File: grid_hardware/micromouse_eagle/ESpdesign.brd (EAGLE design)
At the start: 89.8 x 61 mm, 8 parts

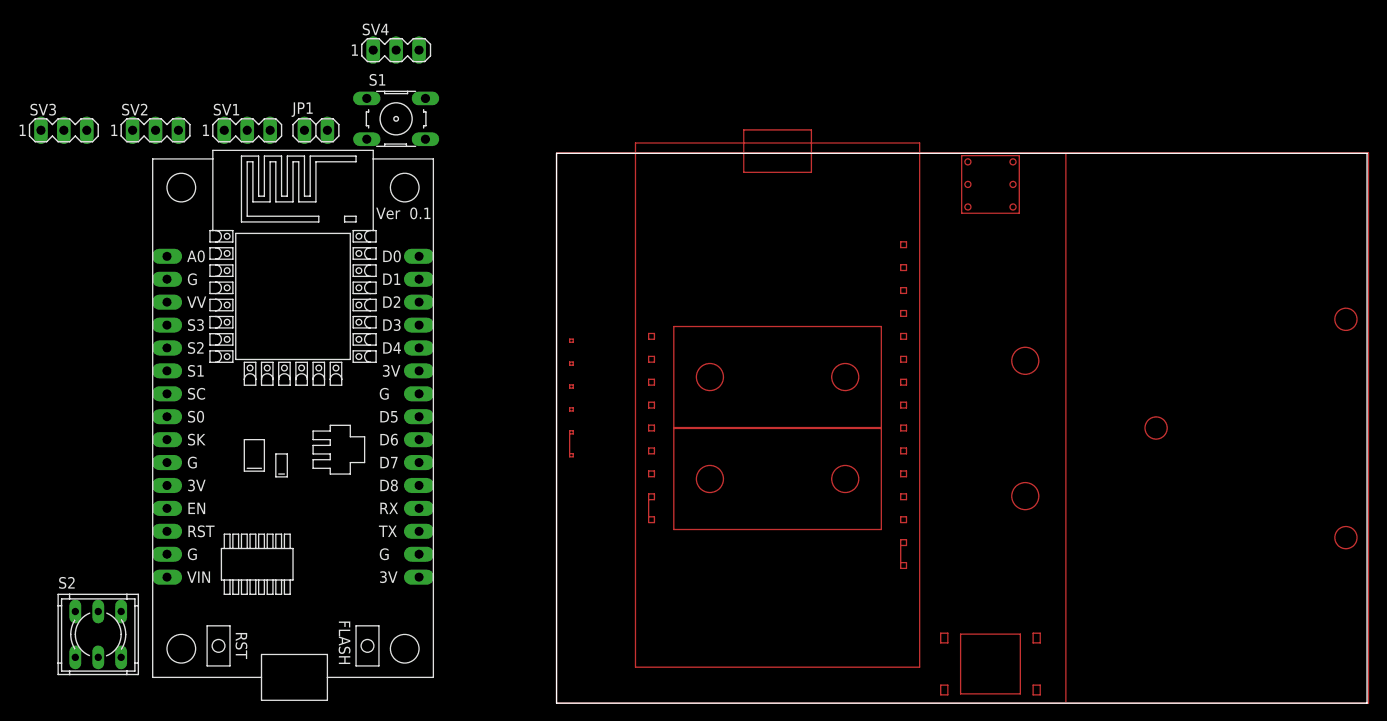
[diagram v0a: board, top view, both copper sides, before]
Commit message: brd continue
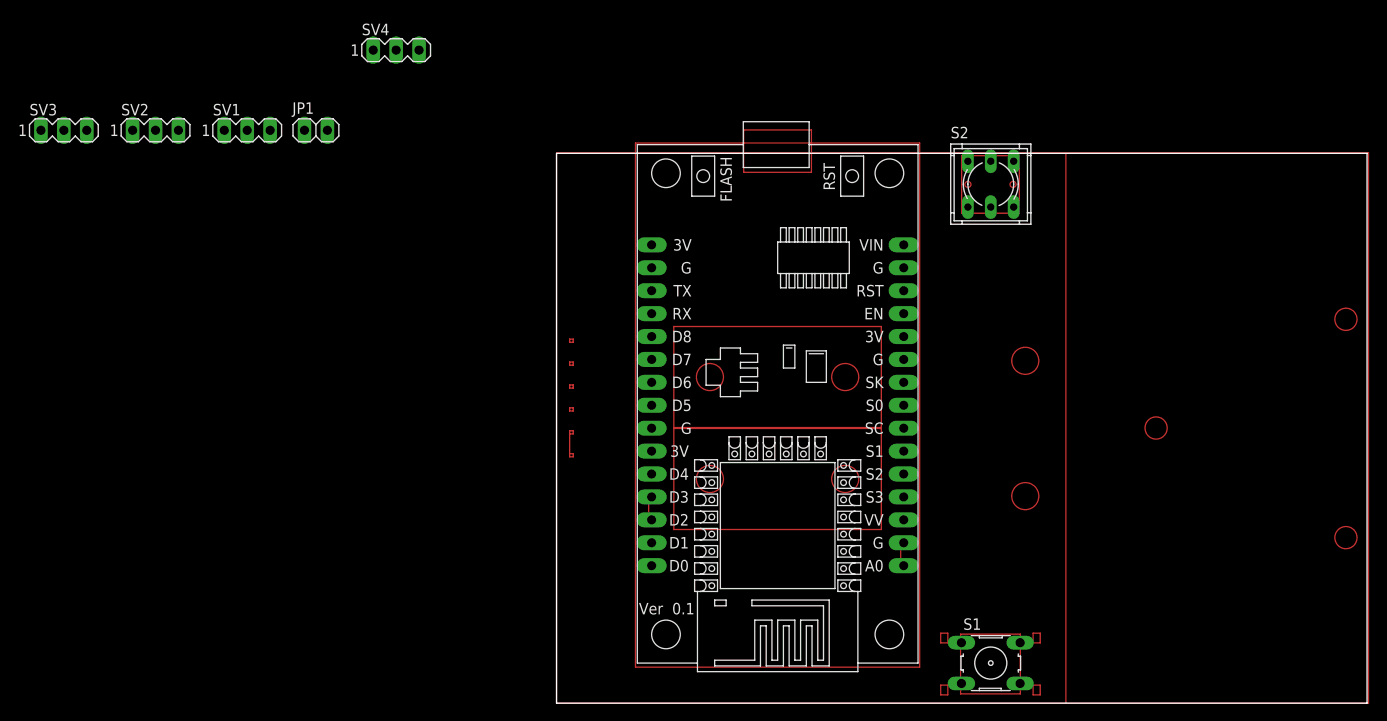
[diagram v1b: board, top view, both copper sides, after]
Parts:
- moved S2 110.8 mm to (48.1, 57.5)
- moved S1 89.4 mm to (48.1, 4.45)
- moved U$1 53.7 mm to (24.5, 33.0), turned to 180 degrees
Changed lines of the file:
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@@
 <attribute name="VALUE" x="-29.21" y="60.325" size="1.27" layer="27"/>
 </element>
-<element name="S1" library="switch-omron" library_urn="urn:adsk.eagle:library:377" package="B3F-10XX" package3d_urn="urn:adsk.eagle:package:27496/1" value="" x="-17.78" y="64.77" smashed="yes">
-<attribute name="MF" value="" x="0" y="0" size="1.778" layer="27" display="off"/>
-<attribute name="MPN" value="B3F-1000" x="0" y="0" size="1.778" layer="27" display="off"/>
-<attribute name="NAME" x="-20.828" y="68.453" size="1.27" layer="25" ratio="10"/>
-<attribute name="OC_FARNELL" value="176432" x="0" y="0" size="1.778" layer="27" display="off"/>
-<attribute name="OC_NEWARK" value="36M3542" x="0" y="0" size="1.778" layer="27" display="off"/>
-<attribute name="POPULARITY" value="72" x="0" y="0" size="1.778" layer="27" display="off"/>
-<attribute name="VALUE" x="-20.828" y="59.69" size="1.27" layer="27" ratio="10"/>
+<element name="S1" library="switch-omron" library_urn="urn:adsk.eagle:library:377" package="B3F-10XX" package3d_urn="urn:adsk.eagle:package:27496/1" value="" x="48.133" y="4.445" smashed="yes">
+<attribute name="MF" value="" x="65.913" y="-60.325" size="1.778" layer="27" display="off"/>
+<attribute name="MPN" value="B3F-1000" x="65.913" y="-60.325" size="1.778" layer="27" display="off"/>
+<attribute name="NAME" x="45.085" y="8.128" size="1.27" layer="25" ratio="10"/>
+<attribute name="OC_FARNELL" value="176432" x="65.913" y="-60.325" size="1.778" layer="27" display="off"/>
+<attribute name="OC_NEWARK" value="36M3542" x="65.913" y="-60.325" size="1.778" layer="27" display="off"/>
+<attribute name="POPULARITY" value="72" x="65.913" y="-60.325" size="1.778" layer="27" display="off"/>
+<attribute name="VALUE" x="45.085" y="-0.635" size="1.27" layer="27" ratio="10"/>
 </element>
-<element name="S2" library="switch-misc-edited" package="9077-2" package3d_urn="urn:adsk.eagle:package:27425/1" value="9077-2" x="-50.8" y="7.62" smashed="yes">
-<attribute name="NAME" x="-55.245" y="12.7" size="1.27" layer="25" ratio="10"/>
-<attribute name="POPULARITY" value="1" x="0" y="0" size="1.778" layer="27" display="off"/>
-<attribute name="VALUE" x="-55.245" y="1.27" size="1.27" layer="27" ratio="10"/>
+<element name="S2" library="switch-misc-edited" package="9077-2" package3d_urn="urn:adsk.eagle:package:27425/1" value="9077-2" x="48.133" y="57.531" smashed="yes">
+<attribute name="NAME" x="43.688" y="62.611" size="1.27" layer="25" ratio="10"/>
+<attribute name="POPULARITY" value="1" x="98.933" y="49.911" size="1.778" layer="27" display="off"/>
+<attribute name="VALUE" x="43.688" y="51.181" size="1.27" layer="27" ratio="10"/>
 </element>
 <element name="SV1" library="con-lstb" library_urn="urn:adsk.eagle:library:162" package="MA03-1" package3d_urn="urn:adsk.eagle:package:8339/1" value="" x="-34.29" y="63.5" smashed="yes">
@@
 <attribute name="VALUE" x="-21.59" y="69.469" size="1.27" layer="27" ratio="10"/>
 </element>
-<element name="U$1" library="nodemcu" package="NODEMCU" value="NODEMCU" x="-29.21" y="31.75" smashed="yes"/>
+<element name="U$1" library="nodemcu" package="NODEMCU" value="NODEMCU" x="24.511" y="33.02" smashed="yes" rot="R180"/>
 </elements>
 <signals>
@@
 <contactref element="S1" pad="1"/>
 <contactref element="S1" pad="2"/>
-<wire x1="-14.5288" y1="67.0306" x2="-17.78" y2="72.39" width="0" layer="19" extent="1-1"/>
-<wire x1="-21.0312" y1="67.0306" x2="-17.78" y2="72.39" width="0" layer="19" extent="1-1"/>
-<wire x1="-43.18" y1="46.99" x2="-21.0312" y2="67.0306" width="0" layer="19" extent="1-1"/>
-<wire x1="-43.18" y1="26.67" x2="-43.18" y2="46.99" width="0" layer="19" extent="1-1"/>
-<wire x1="-43.18" y1="16.51" x2="-43.18" y2="26.67" width="0" layer="19" extent="1-1"/>
-<wire x1="-57.15" y1="63.5" x2="-43.18" y2="46.99" width="0" layer="19" extent="1-1"/>
-<wire x1="-15.24" y1="16.51" x2="-43.18" y2="16.51" width="0" layer="19" extent="1-1"/>
-<wire x1="-15.24" y1="34.29" x2="-15.24" y2="16.51" width="0" layer="19" extent="1-1"/>
+<wire x1="38.481" y1="38.1" x2="38.481" y2="48.26" width="0" layer="19" extent="1-1"/>
+<wire x1="38.481" y1="17.78" x2="38.481" y2="38.1" width="0" layer="19" extent="1-1"/>
+<wire x1="10.541" y1="48.26" x2="38.481" y2="48.26" width="0" layer="19" extent="1-1"/>
+<wire x1="10.541" y1="30.48" x2="10.541" y2="48.26" width="0" layer="19" extent="1-1"/>
+<wire x1="51.3842" y1="6.7056" x2="10.541" y2="48.26" width="0" layer="19" extent="1-1"/>
+<wire x1="-17.78" y1="72.39" x2="51.3842" y2="6.7056" width="0" layer="19" extent="1-1"/>
+<wire x1="44.8818" y1="6.7056" x2="-17.78" y2="72.39" width="0" layer="19" extent="1-1"/>
+<wire x1="-57.15" y1="63.5" x2="44.8818" y2="6.7056" width="0" layer="19" extent="1-1"/>
 </signal>
 <signal name="3V">
@@
 <contactref element="U$1" pad="16"/>
 <contactref element="U$1" pad="25"/>
-<wire x1="-15.24" y1="13.97" x2="-43.18" y2="24.13" width="0" layer="19" extent="1-1"/>
-<wire x1="-15.24" y1="36.83" x2="-15.24" y2="13.97" width="0" layer="19" extent="1-1"/>
+<wire x1="10.541" y1="50.8" x2="38.481" y2="40.64" width="0" layer="19" extent="1-1"/>
+<wire x1="10.541" y1="27.94" x2="10.541" y2="50.8" width="0" layer="19" extent="1-1"/>
 </signal>
 <signal name="D1">
 <contactref element="U$1" pad="29"/>
 <contactref element="SV1" pad="3"/>
-<wire x1="-15.24" y1="46.99" x2="-31.75" y2="63.5" width="0" layer="19" extent="1-1"/>
+<wire x1="10.541" y1="17.78" x2="-31.75" y2="63.5" width="0" layer="19" extent="1-1"/>
 </signal>
 <signal name="5V">
@@
 <contactref element="SV3" pad="2"/>
 <contactref element="JP1" pad="2"/>
+<wire x1="-25.4" y1="63.5" x2="38.481" y2="50.8" width="0" layer="19" extent="1-1"/>
 <wire x1="-54.61" y1="63.5" x2="-25.4" y2="63.5" width="0" layer="19" extent="1-1"/>
-<wire x1="-43.18" y1="13.97" x2="-54.61" y2="63.5" width="0" layer="19" extent="1-1"/>
 </signal>
 <signal name="D8">
 <contactref element="U$1" pad="20"/>
 <contactref element="SV3" pad="3"/>
-<wire x1="-15.24" y1="24.13" x2="-52.07" y2="63.5" width="0" layer="19" extent="1-1"/>
+<wire x1="-52.07" y1="63.5" x2="10.541" y2="40.64" width="0" layer="19" extent="1-1"/>
 </signal>
 <signal name="D7">
@@
 <contactref element="U$1" pad="22"/>
 <contactref element="SV2" pad="1"/>
-<wire x1="-15.24" y1="29.21" x2="-46.99" y2="63.5" width="0" layer="19" extent="1-1"/>
+<wire x1="-46.99" y1="63.5" x2="10.541" y2="35.56" width="0" layer="19" extent="1-1"/>
 </signal>
 <signal name="D5">
 <contactref element="U$1" pad="23"/>
 <contactref element="SV2" pad="2"/>
-<wire x1="-15.24" y1="31.75" x2="-44.45" y2="63.5" width="0" layer="19" extent="1-1"/>
+<wire x1="-44.45" y1="63.5" x2="10.541" y2="33.02" width="0" layer="19" extent="1-1"/>
 </signal>
 <signal name="D4">
 <contactref element="U$1" pad="26"/>
 <contactref element="SV2" pad="3"/>
-<wire x1="-41.91" y1="63.5" x2="-15.24" y2="39.37" width="0" layer="19" extent="1-1"/>
+<wire x1="-41.91" y1="63.5" x2="10.541" y2="25.4" width="0" layer="19" extent="1-1"/>
 </signal>
 <signal name="D3">
 <contactref element="U$1" pad="27"/>
 <contactref element="SV1" pad="1"/>
-<wire x1="-15.24" y1="41.91" x2="-36.83" y2="63.5" width="0" layer="19" extent="1-1"/>
+<wire x1="-36.83" y1="63.5" x2="10.541" y2="22.86" width="0" layer="19" extent="1-1"/>
 </signal>
 <signal name="P+">
@@
 <contactref element="JP1" pad="1"/>
 <wire x1="-27.94" y1="63.5" x2="-15.24" y2="72.39" width="0" layer="19" extent="1-1"/>
-<wire x1="-50.8" y1="10.16" x2="-27.94" y2="63.5" width="0" layer="19" extent="1-1"/>
-<wire x1="-53.34" y1="10.16" x2="-50.8" y2="10.16" width="0" layer="19" extent="1-1"/>
+<wire x1="48.133" y1="60.071" x2="-27.94" y2="63.5" width="0" layer="19" extent="1-1"/>
+<wire x1="45.593" y1="60.071" x2="48.133" y2="60.071" width="0" layer="19" extent="1-1"/>
 </signal>
 <signal name="B-">
@@
 <contactref element="S1" pad="3"/>
 <contactref element="S1" pad="4"/>
-<wire x1="-21.0312" y1="62.5094" x2="-20.32" y2="72.39" width="0" layer="19" extent="1-1"/>
-<wire x1="-14.5288" y1="62.5094" x2="-21.0312" y2="62.5094" width="0" layer="19" extent="1-1"/>
+<wire x1="44.8818" y1="2.1844" x2="-20.32" y2="72.39" width="0" layer="19" extent="1-1"/>
+<wire x1="51.3842" y1="2.1844" x2="44.8818" y2="2.1844" width="0" layer="19" extent="1-1"/>
 </signal>
 <signal name="D2">
 <contactref element="U$1" pad="28"/>
 <contactref element="SV1" pad="2"/>
-<wire x1="-15.24" y1="44.45" x2="-34.29" y2="63.5" width="0" layer="19" extent="1-1"/>
+<wire x1="-34.29" y1="63.5" x2="10.541" y2="20.32" width="0" layer="19" extent="1-1"/>
 </signal>
 <signal name="N$1">
